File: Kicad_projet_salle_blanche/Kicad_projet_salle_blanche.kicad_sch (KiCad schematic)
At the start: 6 parts, among them IC1 HDC3120QDEFRQ1, J1 Conn_01x05_Pin, U2 TPS7A2050PDBVR

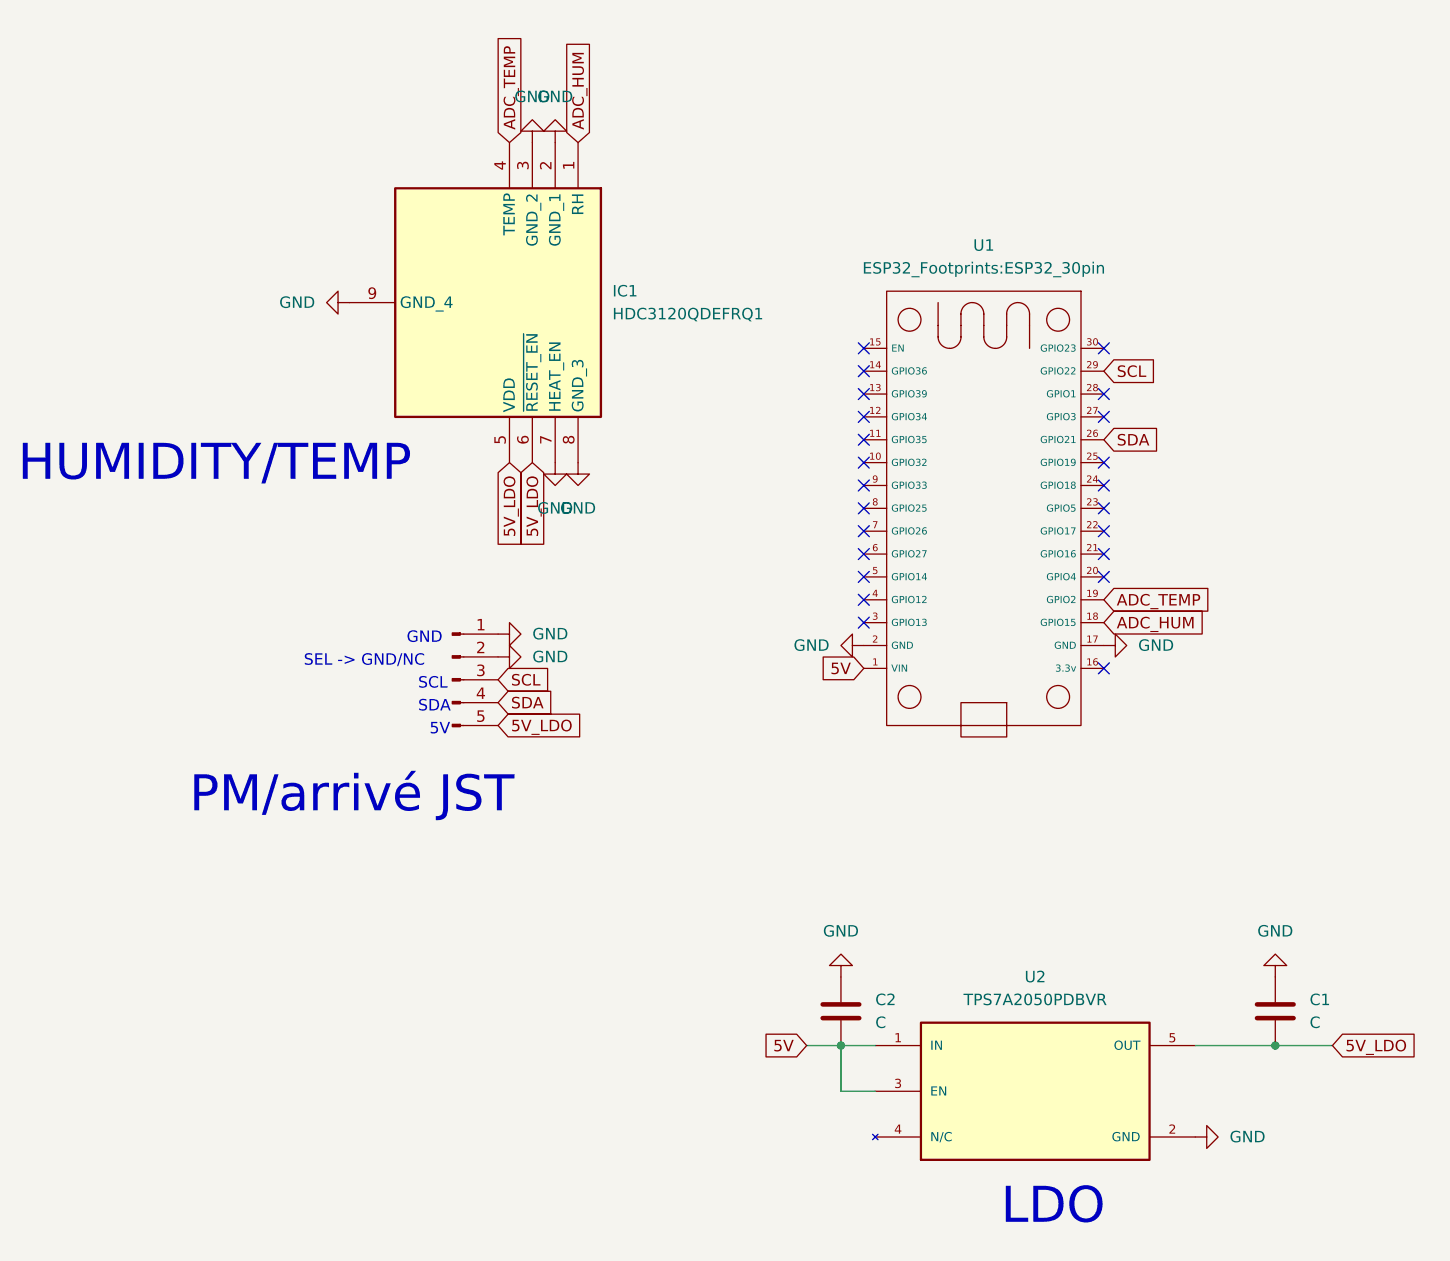
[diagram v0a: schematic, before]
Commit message: 4 pcb terminé
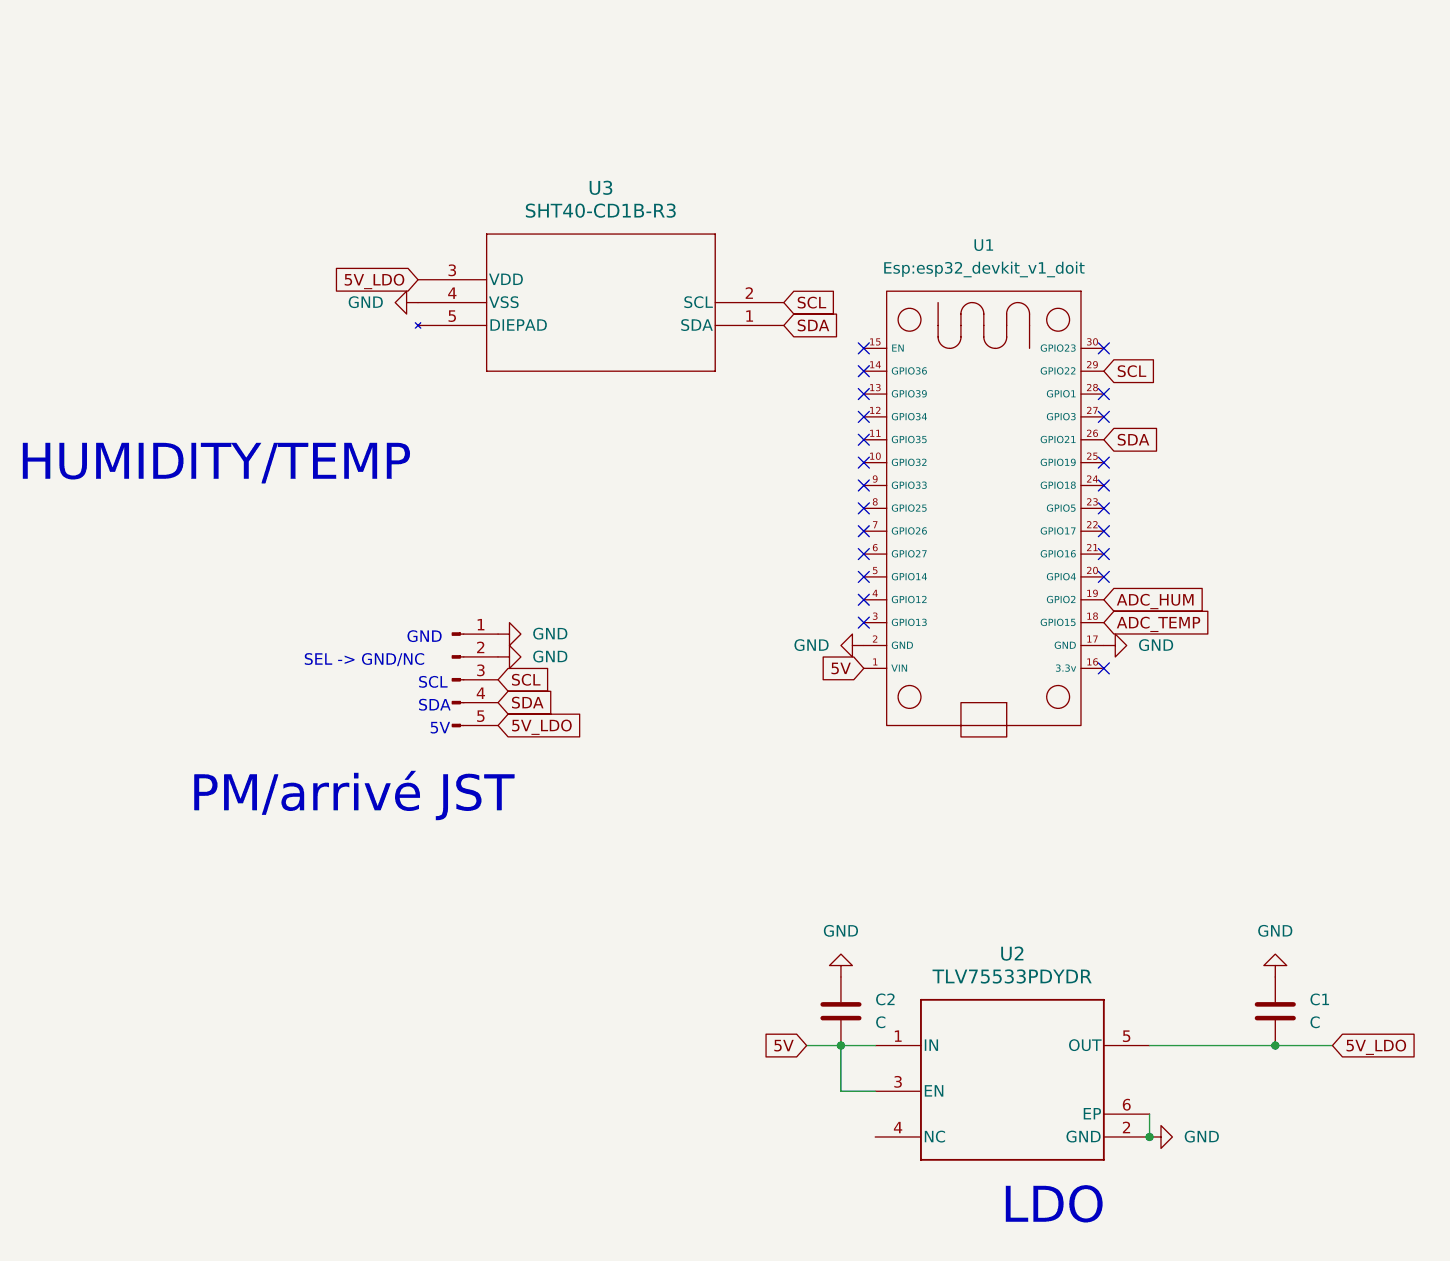
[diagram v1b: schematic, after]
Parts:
- removed IC1: HDC3120QDEFRQ1, TPS7...:SON50P250X250X80-9N-D, symbol HDC3120QDEFRQ1:HDC3120QDEFRQ1
- removed U2: TPS7A2050PDBVR, TPS7...:SON50P250X250X80-9N-D, symbol TPS7A2050PDBVR:TPS7A2050PDBVR
- added U2: TLV75533PDYDR, Esp:DBV0005A-MFG, symbol TLV75533PDYDR:TLV75533PDYDR
- added U3: SHT40-CD1B-R3, Esp:U_SHT3_SEN, symbol SHT40-CD1B-R3:SHT40-CD1B-R3
- J1: footprint Connector_JST:JST_AUH_BM05B-AUHKS-GA-TB_1x05-1MP_P1.50mm_Vertical -> Connector_PinHeader_2.54mm:PinHeader_1x05_P2.54mm_Vertical
- U1: footprint ESP32_Footprints:ESP32_30pin -> Esp:esp32_devkit_v1_doit
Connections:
- net 5V: now also U2.1 (IN), U2.3 (EN)
- net 5V_LDO: now also U2.5 (OUT), U3.3 (VDD)
- net ADC_HUM: now also U1.19 (GPIO2); no longer U1.18 (GPIO15)
- net ADC_TEMP: now also U1.18 (GPIO15); no longer U1.19 (GPIO2)
- net GND: now also U2.2 (GND), U2.6 (EP), U3.4 (VSS)
- net SCL: now also U3.2 (SCL)
- net SDA: now also U3.1 (SDA)
